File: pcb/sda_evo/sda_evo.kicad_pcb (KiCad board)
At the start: 4 copper layers, 61.5 x 105.9 mm, 161 parts, among them J1 PROG, J10 SPKR, J11 AudioJack, J2 USB_C_Receptacle_USB2.0, J3 LCD_CONN, J4 INT_EXP, J5 BATT, J9 Micro_SD_Card_Det, Q1 IRLML6302, SW1 RESET, SW2 BTN_A, SW3 BTN_B, SW4 BTN_UP, SW5 BTN_DOWN, SW6 BTN_LEFT, SW7 BTN_RIGHT, SW8 BTN_PWR, U1 USBLC6, U10 STM32H743ZITx, U11 USBLC6, U12 AP22802AW5-7, U13 LM4861, U2 TLV431, U3 USBLC6, U4 AP22802AW5-7, U5 FT230XS, U6 MCP73831-2-OT, U7 PCM5102, U8 NCP1529, U9 LMR62014XMF, Y1 16Mhz, Y2 32.768

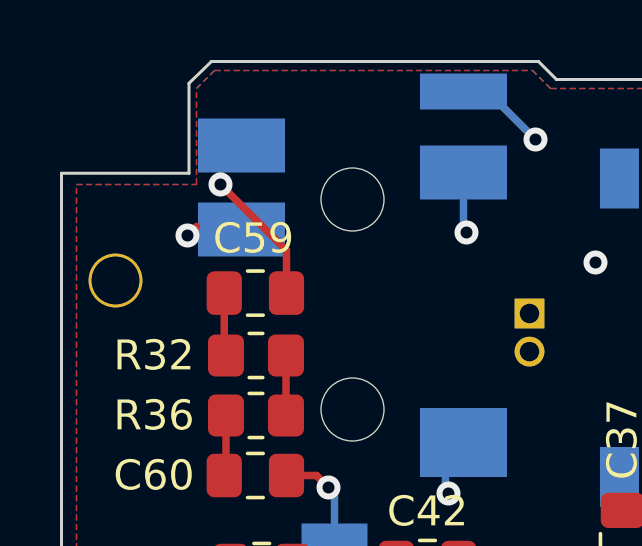
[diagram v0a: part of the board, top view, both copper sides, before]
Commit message: commit before beta1
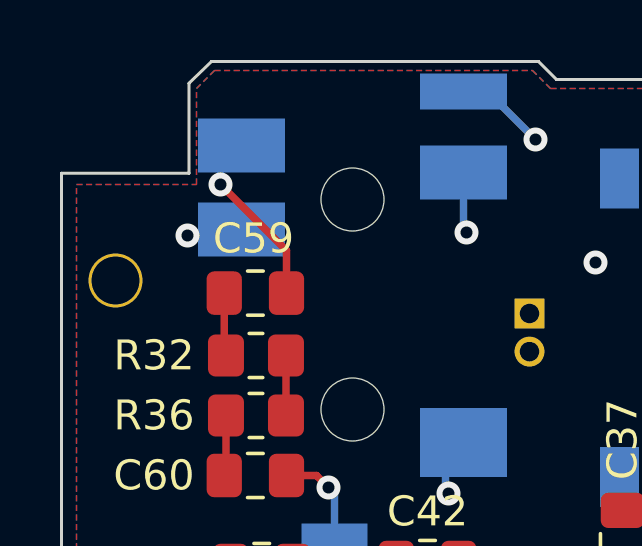
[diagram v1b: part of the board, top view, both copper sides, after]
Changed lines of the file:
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@@
 		)
 		(property "Footprint" "sda-parts:SMDXT224"
-			(at 0 0 -90)
+			(at 0 0 90)
 			(layer "F.Fab")
 			(hide yes)
@@
 		)
 		(property "Datasheet" ""
-			(at 0 0 -90)
+			(at 0 0 90)
 			(layer "F.Fab")
 			(hide yes)
@@
 		)
 		(property "Description" ""
-			(at 0 0 -90)
+			(at 0 0 90)
 			(layer "F.Fab")
 			(hide yes)
@@
 		(width 0.25)
 		(layer "F.Cu")
-		(net 20)
-	)
-	(segment
-		(start 63 53.8)
-		(end 62.7 54.1)
-		(width 0.25)
-		(layer "F.Cu")
